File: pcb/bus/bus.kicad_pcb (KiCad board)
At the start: 4 copper layers, 121.9 x 128.6 mm, 27 parts, among them J201 Conn_02x10_Row_Letter_First, J301 Conn_02x10_Row_Letter_First, J401 Conn_02x10_Row_Letter_First, J501 Conn_02x10_Row_Letter_First, J601 Conn_02x10_Row_Letter_First, J701 Conn_02x10_Row_Letter_First, U101 USBLC6-2SC6, U102 FE1.1s, Y101 12MHz

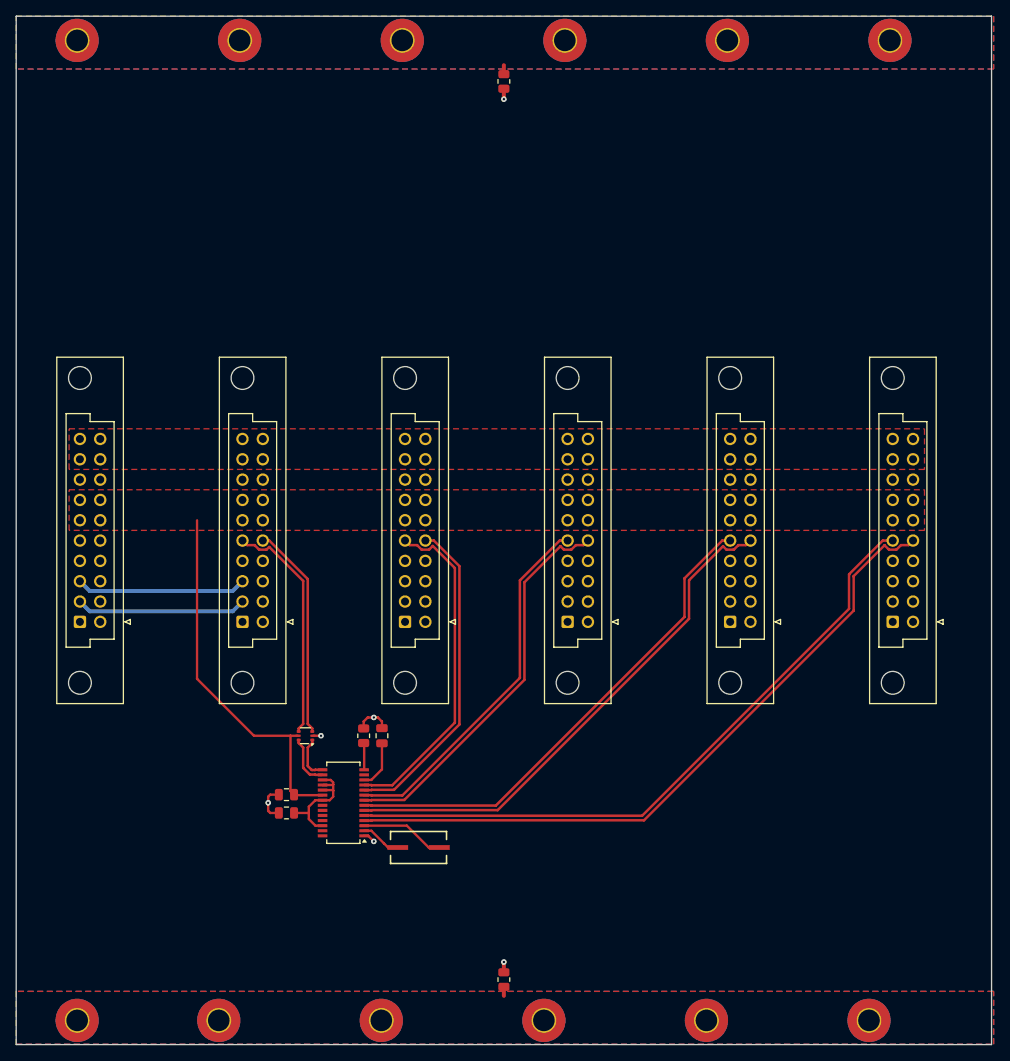
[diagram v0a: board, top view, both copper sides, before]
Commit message: update bus pcb
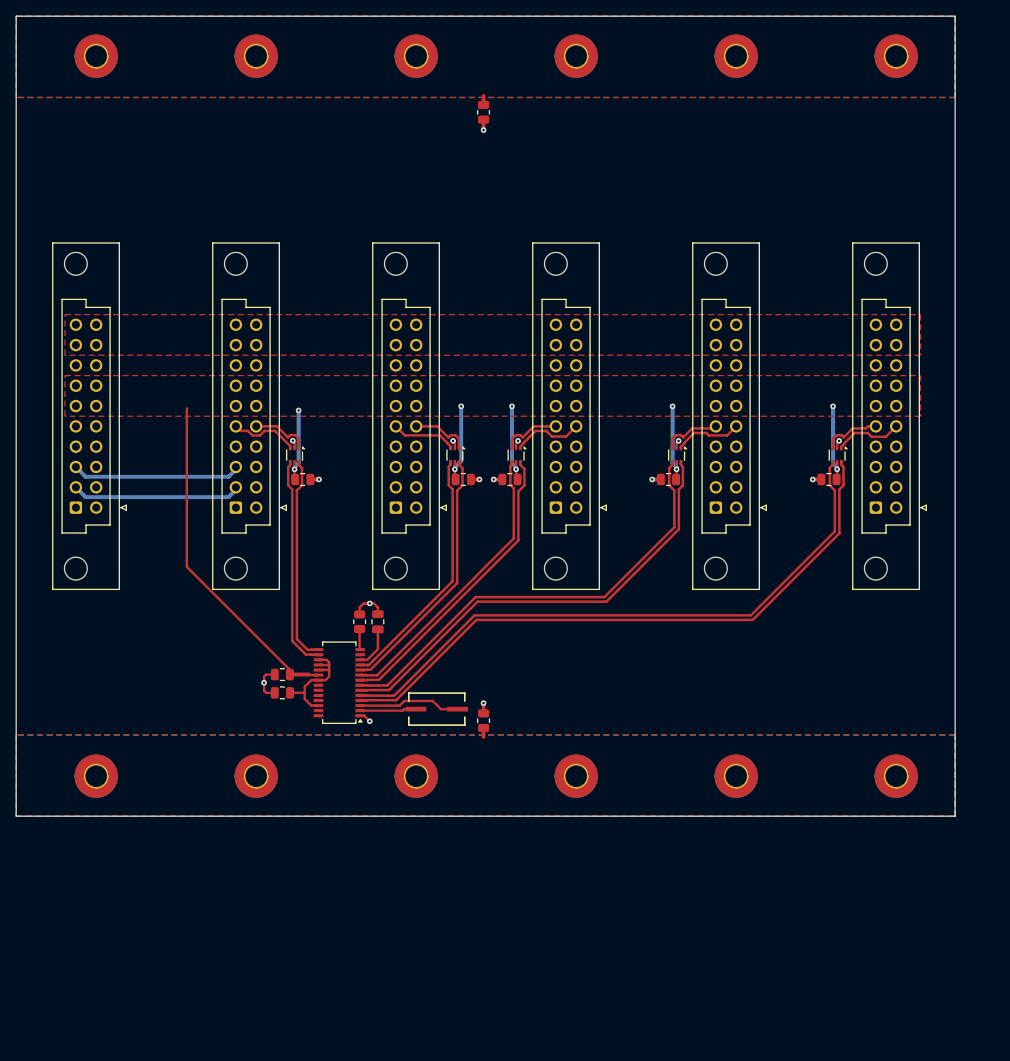
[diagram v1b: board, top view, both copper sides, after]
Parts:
- added C104: 100nF, Capacitor_SMD:C_0805_2012Metric, F.Cu at (101.1, 83.3)
- added C105: 100nF, Capacitor_SMD:C_0805_2012Metric, F.Cu at (121.2, 83.3)
- added C106: 100nF, Capacitor_SMD:C_0805_2012Metric, F.Cu at (127.0, 83.3)
- added C107: 100nF, Capacitor_SMD:C_0805_2012Metric, F.Cu at (146.8, 83.3)
- added C108: 100nF, Capacitor_SMD:C_0805_2012Metric, F.Cu at (166.9, 83.3)
- added U103: USBLC6-2SC6, Package_TO_SOT_SMD:SOT-666, F.Cu at (120.1, 80.3)
- added U104: USBLC6-2SC6, Package_TO_SOT_SMD:SOT-666, F.Cu at (127.8, 80.3)
- added U105: USBLC6-2SC6, Package_TO_SOT_SMD:SOT-666, F.Cu at (147.8, 80.3)
- added U106: USBLC6-2SC6, Package_TO_SOT_SMD:SOT-666, F.Cu at (167.9, 80.3)
- moved U101 35.1 mm to (100.1, 80.3), turned to -90 degrees
- moved R102 32.5 mm to (123.7, 113.5)
- moved H110 30.9 mm to (95.3, 120.4)
- moved H111 30.8 mm to (115.3, 120.4)
- moved H112 30.8 mm to (135.3, 120.4)
- moved H113 30.8 mm to (155.3, 120.4)
- moved H114 30.7 mm to (175.3, 120.4)
- moved H109 30.6 mm to (75.3, 120.4)
- moved Y101 17.4 mm to (117.9, 112.0)
- moved C101 15.0 mm to (98.6, 110.0)
- moved C103 15.0 mm to (98.6, 107.7)
- moved U102 15.0 mm to (105.7, 108.7)
- moved J701 14.4 mm to (175.3, 86.8)
- moved J601 14.4 mm to (155.3, 86.8)
- moved J501 14.4 mm to (135.3, 86.8)
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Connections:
- J201 pad a5: /MASTER_USB+ -> /RPI Connector/NS_USB+
- J201 pad b5: /MASTER_USB- -> /RPI Connector/NS_USB-
- J401 pad a5: /USB1+ -> /Device Connector 1/NS_USB+
- J401 pad b5: /USB1- -> /Device Connector 1/NS_USB-
- J501 pad a5: /USB2+ -> /Device Connector 2/NS_USB+
- J501 pad b5: /USB2- -> /Device Connector 2/NS_USB-
- J601 pad a5: /USB3+ -> /Device Connector 3/NS_USB+
- J601 pad b5: /USB3- -> /Device Connector 3/NS_USB-
- J701 pad a5: /USB4+ -> /Device Connector 4/NS_USB+
- J701 pad b5: /USB4- -> /Device Connector 4/NS_USB-
- U101 pad 1: /MASTER_USB_F- -> /RPI Connector/NS_USB-
- U101 pad 3: /MASTER_USB- -> /RPI Connector/NS_USB+
- U101 pad 6: /MASTER_USB_F+ -> /MASTER_USB-
- U102 pad 15: /MASTER_USB_F- -> /MASTER_USB-
- U102 pad 16: /MASTER_USB_F+ -> /MASTER_USB+
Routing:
- net +5V: track 46.5 -> 89.7 mm, vias 0 -> 10
- net /USB2-: track 48.9 -> 37.4 mm
- net /USB1+: track 41.9 -> 31.3 mm
- net /USB2+: track 45.8 -> 36.1 mm
- net GND: track 14.2 -> 23.4 mm, vias 6 -> 15
- net /Device Connector 2/NS_USB-: track 0.00 -> 8.85 mm
- net /RPI Connector/NS_USB+: track 0.00 -> 8.56 mm
- net /Device Connector 4/NS_USB-: track 0.00 -> 8.54 mm
- net /USB3-: track 65.4 -> 56.9 mm
- net /Device Connector 3/NS_USB-: track 0.00 -> 8.46 mm
- net /USB1-: track 40.7 -> 32.2 mm
- net /USB4-: track 86.1 -> 77.8 mm
- net /Device Connector 1/NS_USB+: track 0.00 -> 8.13 mm
- net /Device Connector 2/NS_USB+: track 0.00 -> 7.55 mm
- net /Device Connector 3/NS_USB+: track 0.00 -> 7.48 mm
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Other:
- board size 121.9 x 128.6 mm -> 117.4 x 100 mm
